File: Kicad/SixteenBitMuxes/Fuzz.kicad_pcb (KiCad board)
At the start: 2 copper layers, 100 x 82 mm, 104 parts, among them J1 Audio In/Out JST XH, J10 JST XH Buttons, J11 LCD JST XH, J12 Bypass Switch JST XH, J2 TONE_POTS, J4 VOL POT A100K JST XH, J5 PowerTest_PinHeader, J6 9V Power JST XH, J7 Boot Reset PinHeader, J9 SWD_PinHeader, Q1 PN2222A, Q10 2SC1815, Q11 PN2222A, Q12 S9013, Q13 MMBT3904, Q14 S9018, Q15 BC848B, Q16 2SC1623, Q17 MPSA18, Q18 MMBT5551L, Q19 2N5088, Q2 MMBT3904, Q20 MMBTA42, Q21 BC807, Q22 BC846, Q23 BC847B, Q24 BC847C, Q25 BC848B, Q26 S9013, Q27 S9018, Q28 C945, Q29 2SC1623, Q3 MMBT5551L, Q30 2SC1815, Q31 MPSA18, Q32 2N5088, Q4 MMBTA42, Q5 BC807, Q6 BC846, Q7 BC847B, Q8 BC847C, Q9 C945, U1 AMS1117-5.0, U2 AMS1117-3.3, U21 CD4051B, U22 4504, U23 4504, U24 4504, U25 CD4053B, U3 STM32F103C8Tx, U4 CD4051B, U6 CD4067BM, U7 CD4067BM, U8 CD4067BM, U9 CD4067BM, Y1 8MHz

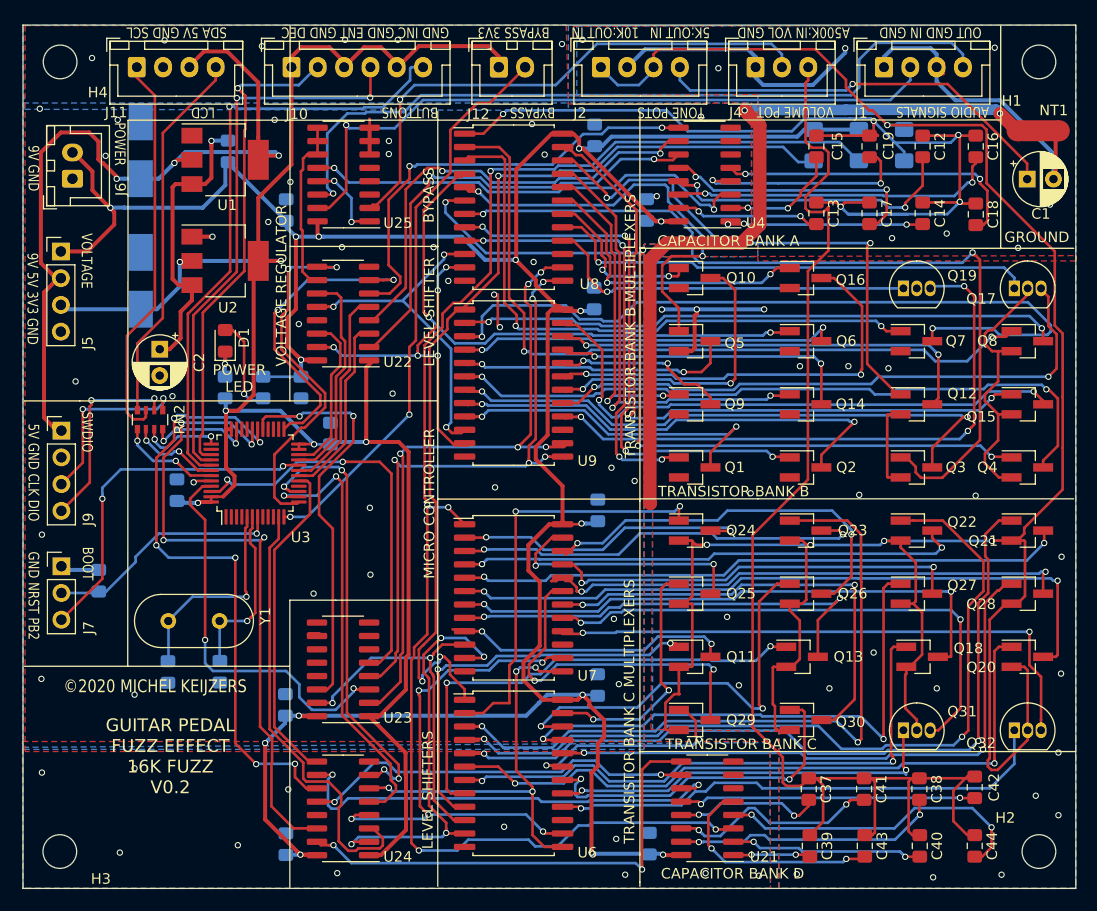
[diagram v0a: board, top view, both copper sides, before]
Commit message: Improvements according video youtube
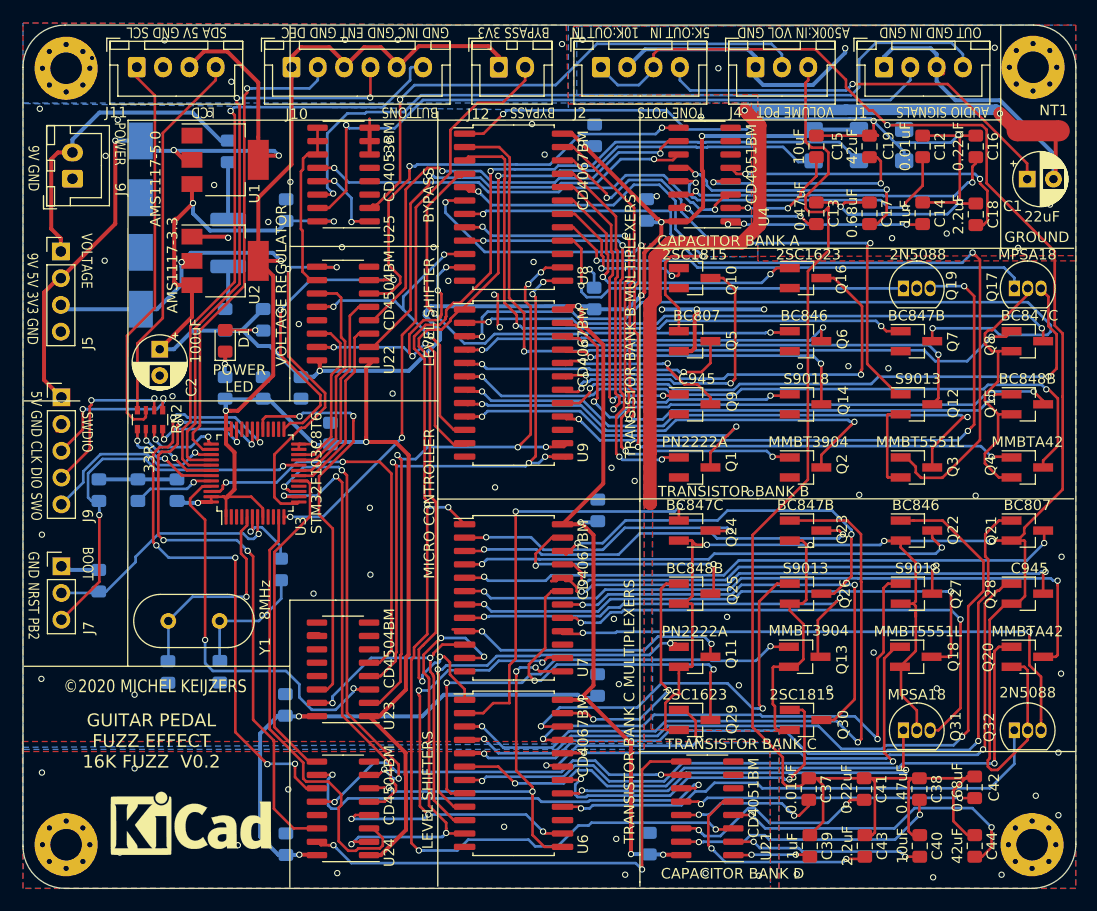
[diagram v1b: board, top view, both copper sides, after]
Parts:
- added C20: 10uF, Capacitor_SMD:C_0805_2012Metric_Pad1.15x1.40mm_HandSolder, B.Cu at (52.8, 64.5)
- added F1: 1.1A(1812), Inductor_SMD:L_1812_4532Metric_Pad1.30x3.40mm_HandSolder, B.Cu at (49.5, 50.7)
- added FB1: 1K/100MHz, Inductor_SMD:L_0805_2012Metric_Pad1.15x1.40mm_HandSolder, B.Cu at (49.2, 58.0)
- added R5: 220R, Resistor_SMD:R_0805_2012Metric_Pad1.15x1.40mm_HandSolder, B.Cu at (54.5, 81.7)
- added R6: 10K, Resistor_SMD:R_0805_2012Metric_Pad1.15x1.40mm_HandSolder, B.Cu at (40.9, 74.2)
- added R7: 10K, Resistor_SMD:R_0805_2012Metric_Pad1.15x1.40mm_HandSolder, B.Cu at (37.2, 74.2)
- added REF**: KiCad-Logo_6mm_SilkScreen, Symbol:KiCad-Logo_6mm_SilkScreen, F.Cu at (46.0, 105.8)
- H1, H2, H3, H4: value MountingHole -> MountingHole_Pad; footprint MountingHole:MountingHole_3.2mm_M3 -> MountingHole:MountingHole_3mm_Pad_Via
- J9: value SWD_PinHeader -> SWD PinHeader; footprint Connector_PinHeader_2.54mm:PinHeader_1x04_P2.54mm_Vertical -> Connector_PinHeader_2.54mm:PinHeader_1x05_P2.54mm_Vertical
- RN2: value R_Pack04 -> 33R
- U21, U4: value CD4051B -> CD4051BM
- U22, U23, U24: value 4504 -> CD4504BM
- U25: value CD4053B -> CD4053BM
- U3: value STM32F103C8Tx -> STM32F103C8T6
- Y1: footprint Crystal:Crystal_HC49-U_Vertical -> Crystal:Crystal_HC49-4H_Vertical
- moved H1 92.4 mm to (34.1, 34.1)
- moved H3 92.4 mm to (125.8, 107.8)
- moved H2 74.5 mm to (125.9, 34.0)
- moved H4 74.4 mm to (34.1, 107.8)
- moved R4 6.43 mm to (52.8, 58.0)
- moved J9 3.16 mm to (33.6, 65.4)
- moved C3 1.81 mm to (41.2, 43.7), turned to 270 degrees
- moved Q18 0.60 mm to (114.8, 90.0)
- moved Q13 0.25 mm to (104.2, 90.0)
- turned D2 to 90 degrees
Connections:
- net /Mcu/PB2 renamed /Mcu/BOOT1
- net Net-(C5-Pad1) renamed /Mcu/OSC_IN
- C11 pad 1: +9V -> /+9V_SAFE
- C2 pad 1: Net-(C2-Pad1) -> /+9V_SAFE
- C21 pad 1: +9V -> /+9V_SAFE
- C22 pad 1: +9V -> /+9V_SAFE
- C23 pad 1: +9V -> /+9V_SAFE
- C24 pad 1: +9V -> /+9V_SAFE
- C36 pad 1: +9V -> /+9V_SAFE
- C45 pad 1: +9V -> /+9V_SAFE
- C46 pad 1: +9V -> /+9V_SAFE
- C47 pad 1: +9V -> /+9V_SAFE
- C48 pad 1: +9V -> /+9V_SAFE
- D2 pad 1: Net-(C2-Pad1) -> Net-(D2-Pad1)
- H1 pad 1: (no net) -> GND
- H2 pad 1: (no net) -> GNDA
- H3 pad 1: (no net) -> GNDA
- H4 pad 1: (no net) -> GND
- R1 pad 1: +9V -> /+9V_SAFE
- R3 pad 1: +9V -> /+9V_SAFE
- R4 pad 1: +9V -> /+9V_SAFE
- U1 pad 3: Net-(C2-Pad1) -> /+9V_SAFE
- U2 pad 3: Net-(C2-Pad1) -> /+9V_SAFE
- U21 pad 16: +9V -> /+9V_SAFE
- U22 pad 16: +9V -> /+9V_SAFE
- U23 pad 16: +9V -> /+9V_SAFE
- U24 pad 16: +9V -> /+9V_SAFE
- U25 pad 16: +9V -> /+9V_SAFE
- U3 pad 1: Net-(U3-Pad1) -> +3V3
- U3 pad 38: Net-(U3-Pad38) -> /Mcu/GPIO_BUTTON_DECREASE
- U3 pad 39: /Mcu/GPIO_BUTTON_DECREASE -> /Mcu/SYS_JTDO_TRACESWO
- U3 pad 44: GND -> Net-(R6-Pad1)
- U3 pad 6: Net-(C6-Pad1) -> /Mcu/OSC_OUT
- U3 pad 8: Net-(U3-Pad8) -> +3V3
- U4 pad 16: +9V -> /+9V_SAFE
- U6 pad 24: +9V -> /+9V_SAFE
- U7 pad 24: +9V -> /+9V_SAFE
- U8 pad 24: +9V -> /+9V_SAFE
- U9 pad 24: +9V -> /+9V_SAFE
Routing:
- net /+9V_SAFE: track 0.00 -> 268.7 mm, vias 0 -> 14
- net +9V: track 279.5 -> 29.6 mm, vias 15 -> 0
- net Net-(C2-Pad1): track 27.9 -> 0.00 mm, vias 1 -> 0
- net /Mcu/SYS_JTDO_TRACESWO: track 0.00 -> 18.3 mm, vias 0 -> 1
- net +5V: track 76.9 -> 64.7 mm
- net +3V3: track 179.1 -> 189.1 mm
- net GND: track 91.2 -> 100.8 mm, vias 55 -> 56
- net Net-(R6-Pad1): track 0.00 -> 7.84 mm, vias 0 -> 1
- net /Mcu/OSC_OUT: track 0.00 -> 6.42 mm, vias 0 -> 1
- net Net-(D1-Pad2): track 9.12 -> 3.62 mm
- net Net-(D2-Pad1): track 0.00 -> 5.45 mm
- net Net-(C6-Pad1): track 17.5 -> 12.9 mm, vias 1 -> 0
- net Net-(F1-Pad2): track 0.00 -> 4.17 mm
- net /Mcu/BOOT1: track 33.7 -> 37.5 mm
- net /Mcu/SYS_JTMS_SWDIO: track 17.4 -> 14.3 mm
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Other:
- outline, holes or cut-outs redrawn
- board text added: "5V GND CLK DIO SWO"
- board text removed: "5V GND CLK DIO"
- board text removed: "VOLTAGE REGULATOR DIODES"
